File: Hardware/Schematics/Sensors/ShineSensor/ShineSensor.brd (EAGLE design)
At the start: 10.2 x 14.9 mm, 7 parts, among them Q1 BSS138

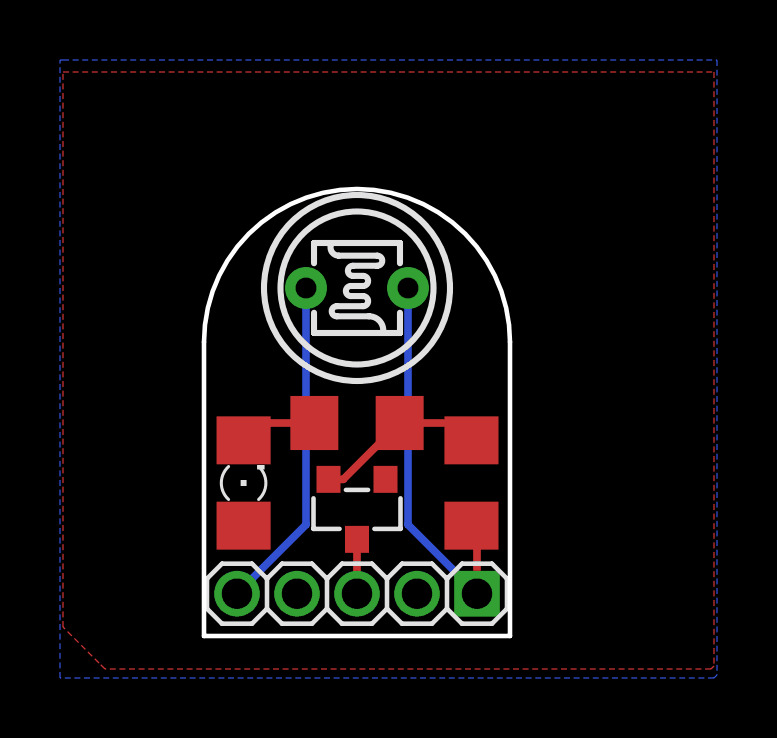
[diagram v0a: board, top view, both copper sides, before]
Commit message: gerber update
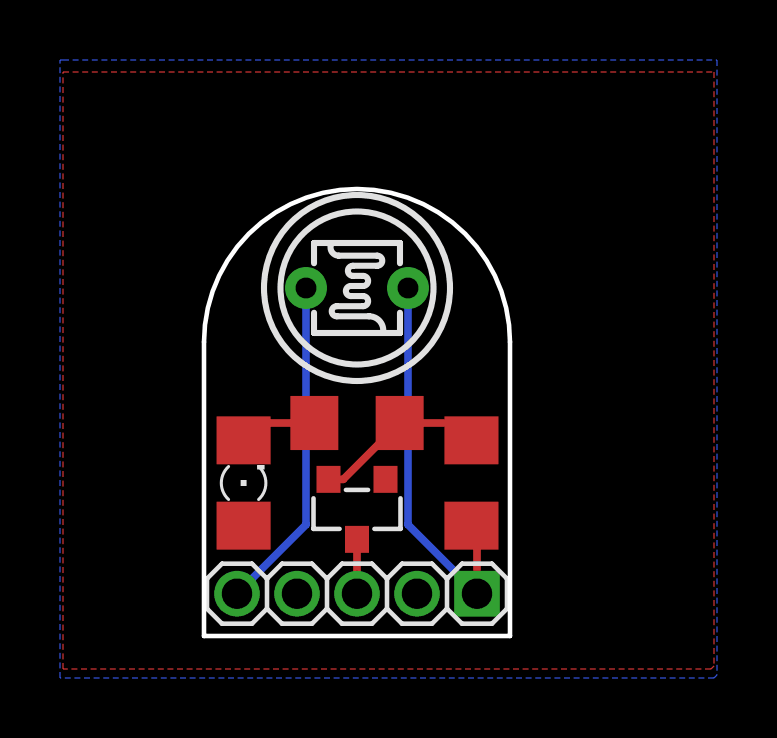
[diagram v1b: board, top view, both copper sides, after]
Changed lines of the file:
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@@
 <drawing>
 <settings>
-<setting alwaysvectorfont="no"/>
+<setting alwaysvectorfont="yes"/>
 <setting keepoldvectorfont="yes"/>
 <setting verticaltext="up"/>
@@
 <vertex x="11.9" y="1.4"/>
 <vertex x="11.8" y="1.3"/>
-<vertex x="-8.4" y="1.3"/>
-<vertex x="-8.6" y="1.5"/>
-<vertex x="-9.8" y="2.7"/>
+<vertex x="-9.8" y="1.3"/>
 </polygon>
 <wire x1="-1.7" y1="14" x2="-1.7" y2="6.11" width="0.254" layer="16"/>
